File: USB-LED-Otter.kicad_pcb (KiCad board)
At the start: 2 copper layers, 12 x 15 mm, 14 parts, among them J1 USB, J2 PAD, J3 LED, J4 PAD, J5 PAD, SW1 DFU, U1 MCP1700-3302E_SOT23, U2 STM32F072C8Ux

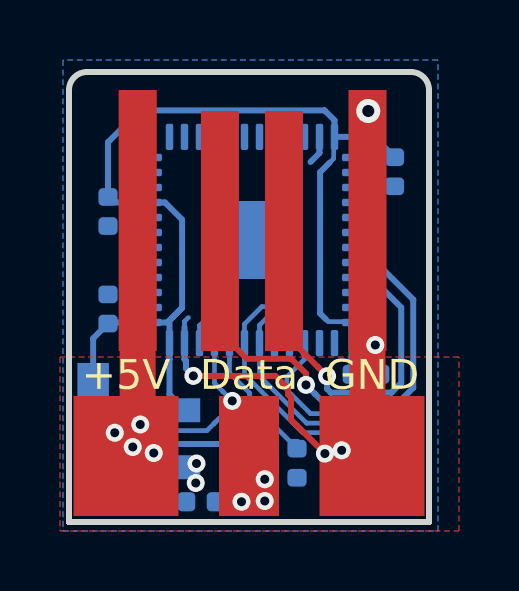
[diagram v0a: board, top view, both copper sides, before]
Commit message: added example code
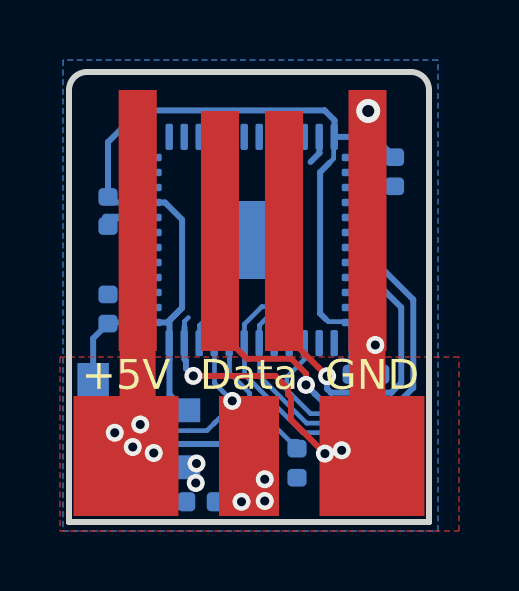
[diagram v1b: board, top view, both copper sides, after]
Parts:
- U2: value STM32F072C8Ux -> STM32F072CBUx
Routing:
- net GND: track 25.1 -> 26.9 mm
